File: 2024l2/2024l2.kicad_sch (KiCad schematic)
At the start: 124 parts, among them IC1 LM2587S-ADJ, J10 Conn_01x03, J11 Conn_01x04, J2 Conn_01x02, J4 Conn_01x02, J5 Conn_01x02, J7 Conn_01x03, J8 Conn_01x06, SW1 SW_SPST, U1 DRV8873SPWPRQ1, U3 TPS5430DDA, U4 TPS5430DDA, U7 Teensy 4.0

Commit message: LCSC Updates
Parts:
- C17, C3, C4: LCSC C577419 -> C3011705
- C29, C31: LCSC C5128349 -> C3011705
- D1, D2: LCSC C6807781 -> C85099
- R19: LCSC C22909 -> C137748
- R2: LCSC C25804 -> C21190
- R2: LCSC C25804 -> C23138
- R2: LCSC C25804 -> C21189
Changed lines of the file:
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@@
       (effects (font (size 1.27 1.27)) hide)
     )
-    (property "LCSC" "C25804" (at 281.94 49.53 0)
+    (property "LCSC" "C21190" (at 281.94 49.53 0)
       (effects (font (size 1.27 1.27)) hide)
     )
@@
       (effects (font (size 1.27 1.27)) hide)
     )
-    (property "LCSC" "C25804" (at 147.32 109.22 0)
+    (property "LCSC" "C21190" (at 147.32 109.22 0)
       (effects (font (size 1.27 1.27)) hide)
     )
@@
       (effects (font (size 1.27 1.27)) hide)
     )
-    (property "LCSC" "C577419" (at 255.27 34.29 0)
+    (property "LCSC" "C3011705" (at 255.27 34.29 0)
       (effects (font (size 1.27 1.27)) hide)
     )
@@
       (effects (font (size 1.27 1.27)) hide)
     )
-    (property "LCSC" "C25804" (at 281.94 115.57 0)
+    (property "LCSC" "C21190" (at 281.94 115.57 0)
       (effects (font (size 1.27 1.27)) hide)
     )
@@
       (effects (font (size 1.27 1.27)) hide)
     )
-    (property "LCSC" "C25804" (at 16.51 238.76 0)
+    (property "LCSC" "C23138" (at 16.51 238.76 0)
       (effects (font (size 1.27 1.27)) hide)
     )
@@
       (effects (font (size 1.27 1.27)) hide)
     )
-    (property "LCSC" "C25804" (at 222.25 116.84 0)
+    (property "LCSC" "C21189" (at 222.25 116.84 0)
       (effects (font (size 1.27 1.27)) hide)
     )
@@
       (effects (font (size 1.27 1.27)) hide)
     )
-    (property "LCSC" "C5128349" (at 331.47 191.77 0)
+    (property "LCSC" "C3011705" (at 331.47 191.77 0)
       (effects (font (size 1.27 1.27)) hide)
     )
@@
       (effects (font (size 1.27 1.27)) hide)
     )
-    (property "LCSC" "C25804" (at 356.87 123.19 0)
+    (property "LCSC" "C21189" (at 356.87 123.19 0)
       (effects (font (size 1.27 1.27)) hide)
     )
@@
       (effects (font (size 1.27 1.27)) hide)
     )
-    (property "LCSC" "C25804" (at 147.32 43.18 0)
+    (property "LCSC" "C21190" (at 147.32 43.18 0)
       (effects (font (size 1.27 1.27)) hide)
     )
@@
       (effects (font (size 1.27 1.27)) hide)
     )
-    (property "LCSC" "C6807781" (at 77.47 26.67 90)
+    (property "LCSC" "C85099" (at 77.47 26.67 90)
       (effects (font (size 1.27 1.27)) hide)
     )
@@
       (effects (font (size 1.27 1.27)) hide)
     )
-    (property "LCSC" "C577419" (at 106.68 72.39 0)
+    (property "LCSC" "C3011705" (at 106.68 72.39 0)
       (effects (font (size 1.27 1.27)) hide)
     )
@@
       (effects (font (size 1.27 1.27)) hide)
     )
-    (property "LCSC" "C25804" (at 222.25 50.8 0)
+    (property "LCSC" "C21189" (at 222.25 50.8 0)
       (effects (font (size 1.27 1.27)) hide)
     )
@@
       (effects (font (size 1.27 1.27)) hide)
     )
-    (property "LCSC" "C6807781" (at 77.47 72.39 90)
+    (property "LCSC" "C85099" (at 77.47 72.39 90)
       (effects (font (size 1.27 1.27)) hide)
     )
@@
       (effects (font (size 1.27 1.27)) hide)
     )
-    (property "LCSC" "C577419" (at 394.97 105.41 0)
+    (property "LCSC" "C3011705" (at 394.97 105.41 0)
       (effects (font (size 1.27 1.27)) hide)
     )
@@
       (effects (font (size 1.27 1.27)) hide)
     )
-    (property "LCSC" "C577419" (at 106.68 26.67 0)
+    (property "LCSC" "C3011705" (at 106.68 26.67 0)
       (effects (font (size 1.27 1.27)) hide)
     )
@@
       (effects (font (size 1.27 1.27)) hide)
     )
-    (property "LCSC" "C25804" (at 16.51 267.97 0)
+    (property "LCSC" "C23138" (at 16.51 267.97 0)
       (effects (font (size 1.27 1.27)) hide)
     )
@@
       (effects (font (size 1.27 1.27)) hide)
     )
-    (property "LCSC" "C5128349" (at 232.41 191.77 0)
+    (property "LCSC" "C3011705" (at 232.41 191.77 0)
       (effects (font (size 1.27 1.27)) hide)
     )
@@
       (effects (font (size 1.27 1.27)) hide)
     )
-    (property "LCSC" "C25804" (at 31.75 269.24 0)
+    (property "LCSC" "C23138" (at 31.75 269.24 0)
       (effects (font (size 1.27 1.27)) hide)
     )
@@
       (effects (font (size 1.27 1.27)) hide)
     )
-    (property "LCSC" "C25804" (at 31.75 238.76 0)
+    (property "LCSC" "C23138" (at 31.75 238.76 0)
       (effects (font (size 1.27 1.27)) hide)
     )
@@
       (effects (font (size 1.27 1.27)) hide)
     )
-    (property "LCSC" "C577419" (at 256.54 100.33 0)
+    (property "LCSC" "C3011705" (at 256.54 100.33 0)
       (effects (font (size 1.27 1.27)) hide)
     )
@@
       (effects (font (size 1.27 1.27)) hide)
     )
-    (property "LCSC" "C25804" (at 356.87 57.15 0)
+    (property "LCSC" "C21189" (at 356.87 57.15 0)
       (effects (font (size 1.27 1.27)) hide)
     )
@@
       (effects (font (size 1.27 1.27)) hide)
     )
-    (property "LCSC" "C22909" (at 256.54 196.85 0)
+    (property "LCSC" "C137748" (at 256.54 196.85 0)
       (effects (font (size 1.27 1.27)) hide)
     )
@@
       (effects (font (size 1.27 1.27)) hide)
     )
-    (property "LCSC" "C577419" (at 394.97 39.37 0)
+    (property "LCSC" "C3011705" (at 394.97 39.37 0)
       (effects (font (size 1.27 1.27)) hide)
     )

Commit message: LCSC
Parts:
- L3: LCSC C7461383 -> C2875750
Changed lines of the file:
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@@
       (effects (font (size 1.27 1.27)) hide)
     )
-    (property "LCSC" "C7461383" (at 279.4 175.26 90)
+    (property "LCSC" "C2875750" (at 279.4 175.26 90)
       (effects (font (size 1.27 1.27)) hide)
     )

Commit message: Move motor switch
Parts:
- RV1: LCSC C124590 -> C3151613
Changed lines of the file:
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@@
       (effects (font (size 1.27 1.27)) hide)
     )
-    (property "LCSC" "C124590" (at 304.8 193.04 90)
+    (property "LCSC" "C3151613" (at 304.8 193.04 90)
       (effects (font (size 1.27 1.27)) hide)
     )

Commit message: Changed Cap LCSC
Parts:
- C3: LCSC C259982 -> C5162352
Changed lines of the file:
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@@
       (effects (font (size 1.27 1.27)) hide)
     )
-    (property "LCSC" "C259982" (at 382.27 39.37 0)
+    (property "LCSC" "C5162352" (at 382.27 39.37 0)
       (effects (font (size 1.27 1.27)) hide)
     )
@@
       (effects (font (size 1.27 1.27)) hide)
     )
-    (property "LCSC" "C259982" (at 243.84 100.33 0)
+    (property "LCSC" "C5162352" (at 243.84 100.33 0)
       (effects (font (size 1.27 1.27)) hide)
     )
@@
       (effects (font (size 1.27 1.27)) hide)
     )
-    (property "LCSC" "C259982" (at 242.57 34.29 0)
+    (property "LCSC" "C5162352" (at 242.57 34.29 0)
       (effects (font (size 1.27 1.27)) hide)
     )
@@
       (effects (font (size 1.27 1.27)) hide)
     )
-    (property "LCSC" "C259982" (at 382.27 105.41 0)
+    (property "LCSC" "C5162352" (at 382.27 105.41 0)
       (effects (font (size 1.27 1.27)) hide)
     )

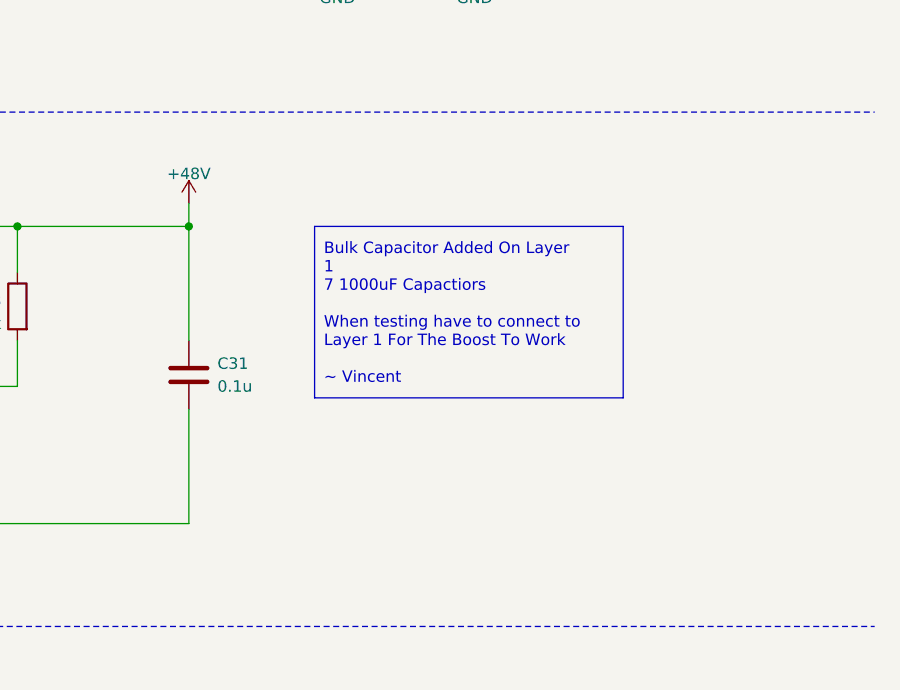
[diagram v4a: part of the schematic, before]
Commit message: Boost Caps
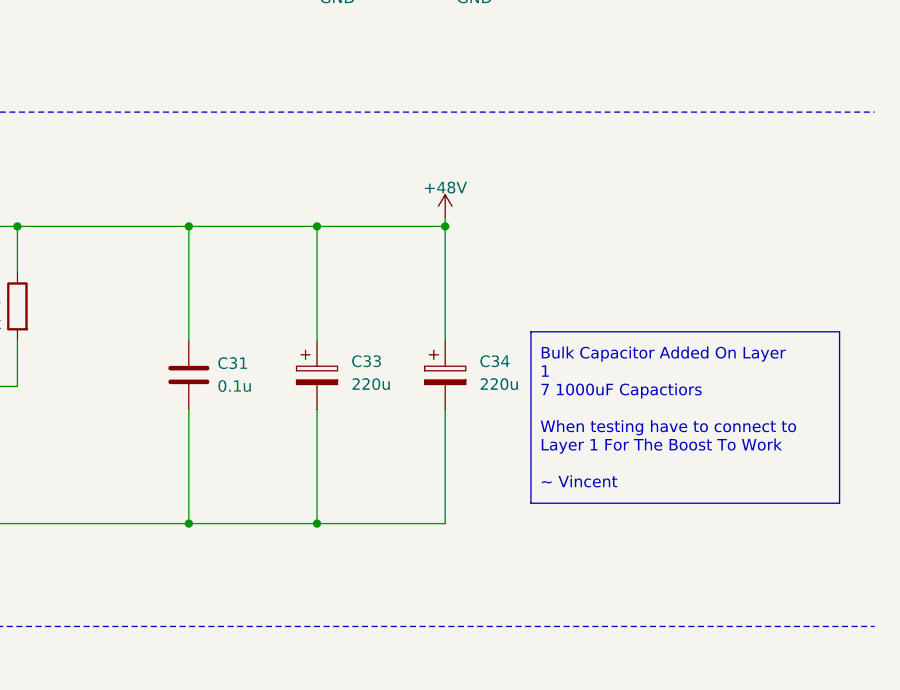
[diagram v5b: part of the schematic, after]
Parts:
- added C33, C34: 220u, Capacitor_SMD:CP_Elec_10x10.5, symbol Device:C_Polarized
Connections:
- net +48V: now also C33.1, C34.1
- net GND: now also C33.2, C34.2
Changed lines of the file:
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@@
   (junction (at 278.13 208.28) (diameter 0) (color 0 0 0 0)
   )
+  (junction (at 345.7119 175.26) (diameter 0) (color 0 0 0 0)
+  )
   (junction (at 347.98 105.41) (diameter 0) (color 0 0 0 0)
   )
@@
   (junction (at 228.6 138.43) (diameter 0) (color 0 0 0 0)
   )
+  (junction (at 359.9536 175.26) (diameter 0) (color 0 0 0 0)
+  )
   (junction (at 243.84 144.78) (diameter 0) (color 0 0 0 0)
   )
@@
   (junction (at 106.68 21.59) (diameter 0) (color 0 0 0 0)
   )
+  (junction (at 345.7119 208.28) (diameter 0) (color 0 0 0 0)
+  )
   (junction (at 92.71 67.31) (diameter 0) (color 0 0 0 0)
   )
@@
   (junction (at 299.72 193.04) (diameter 0) (color 0 0 0 0)
   )
+  (junction (at 331.47 208.28) (diameter 0) (color 0 0 0 0)
+  )
   (junction (at 331.47 175.26) (diameter 0) (color 0 0 0 0)
   )
@@
     (stroke (width 0) (type default))
   )
+  (wire (pts (xy 359.9536 175.26) (xy 359.9538 175.26))
+    (stroke (width 0) (type default))
+  )
   (polyline (pts (xy 12.7 102.87) (xy 127 102.87))
     (stroke (width 0) (type dash))
@@
     (stroke (width 0) (type default))
   )
+  (wire (pts (xy 331.47 208.28) (xy 345.7119 208.28))
+    (stroke (width 0) (type default))
+  )
   (wire (pts (xy 157.48 96.52) (xy 153.67 96.52))
     (stroke (width 0) (type default))
@@
     (stroke (width 0) (type default))
   )
-  (wire (pts (xy 331.47 175.26) (xy 331.47 172.72))
+  (wire (pts (xy 359.9536 175.26) (xy 359.9536 174.2915))
     (stroke (width 0) (type default))
   )
@@
     (stroke (width 0) (type default))
   )
+  (wire (pts (xy 345.7119 175.26) (xy 331.47 175.26))
+    (stroke (width 0) (type default))
+  )
+  (wire (pts (xy 345.7119 175.26) (xy 345.7119 188.0025))
+    (stroke (width 0) (type default))
+  )
   (wire (pts (xy 278.13 208.28) (xy 276.86 208.28))
     (stroke (width 0) (type default))
@@
     (stroke (width 0) (type default))
   )
+  (wire (pts (xy 359.9538 175.26) (xy 359.9538 188.0025))
+    (stroke (width 0) (type default))
+  )
   (wire (pts (xy 255.27 27.94) (xy 255.27 30.48))
     (stroke (width 0) (type default))
@@
     (stroke (width 0) (type default))
   )
+  (wire (pts (xy 345.7119 175.26) (xy 359.9536 175.26))
+    (stroke (width 0) (type default))
+  )
   (wire (pts (xy 299.72 71.12) (xy 309.88 71.12))
     (stroke (width 0) (type default))
@@
     (stroke (width 0) (type default))
   )
+  (wire (pts (xy 345.7119 208.28) (xy 359.9538 208.28))
+    (stroke (width 0) (type default))
+  )
   (wire (pts (xy 77.47 76.2) (xy 77.47 77.47))
     (stroke (width 0) (type default))
@@
     (stroke (width 0) (type default))
   )
+  (wire (pts (xy 359.9538 208.28) (xy 359.9538 195.6225))
+    (stroke (width 0) (type default))
+  )
   (wire (pts (xy 299.72 55.88) (xy 309.88 55.88))
     (stroke (width 0) (type default))
@@
     (stroke (width 0) (type default))
   )
+  (wire (pts (xy 345.7119 208.28) (xy 345.7119 195.6225))
+    (stroke (width 0) (type default))
+  )
   (wire (pts (xy 213.36 87.63) (xy 213.36 90.17))
     (stroke (width 0) (type default))
@@
   )
   (text_box "Bulk Capacitor Added On Layer 1\n7 1000uF Capactiors\n\nWhen testing have to connect to Layer 1 For The Boost To Work\n\n~ Vincent"
-    (at 345.44 175.26 0) (size 34.29 19.05)
+    (at 369.4814 186.9696 0) (size 34.29 19.05)
     (stroke (width 0) (type default))
     (fill (type none))
@@
     )
   )
+  (symbol (lib_id "Device:C_Polarized") (at 345.7119 191.8125 0) (unit 1)
+    (in_bom yes) (on_board yes) (dnp no) (fields_autoplaced)
+    (property "Reference" "C33" (at 349.5219 190.2885 0)
+      (effects (font (size 1.27 1.27)) (justify left))
+    )
+    (property "Value" "220u" (at 349.5219 192.8285 0)
+      (effects (font (size 1.27 1.27)) (justify left))
+    )
+    (property "Footprint" "Capacitor_SMD:CP_Elec_10x10.5" (at 346.6771 195.6225 0)
+      (effects (font (size 1.27 1.27)) hide)
+    )
+    (property "Datasheet" "~" (at 345.7119 191.8125 0)
+      (effects (font (size 1.27 1.27)) hide)
+    )
+    (property "LCSC" "C7471900" (at 345.7119 191.8125 0)
+      (effects (font (size 1.27 1.27)) hide)
+    )
+    (pin "1")
+    (pin "2")
+    (instances
+      (project "2024l2"
+        (path "/36f2ccec-186b-4304-87fe-6495d5655b87"
+          (reference "C33") (unit 1)
+        )
+      )
+      (project "2024l1"
+        (path "/5be543b5-1bdc-438f-a916-f916127c0a2b"
+          (reference "C?") (unit 1)
+        )
+      )
+      (project "2023l1-int"
+        (path "/dd82140d-c14c-4d8d-8674-edeceaca486e"
+          (reference "C?") (unit 1)
+        )
+      )
+      (project "buck"
+        (path "/df3073b9-8d60-44a4-89ea-71f9aa763c80"
+          (reference "C?") (unit 1)
+        )
+      )
+    )
+  )
   (symbol (lib_id "Connector_Generic:Conn_01x03") (at 49.53 133.35 180) (unit 1)
     (in_bom yes) (on_board yes) (dnp no)
@@
     )
   )
+  (symbol (lib_id "Device:C_Polarized") (at 359.9538 191.8125 0) (unit 1)
+    (in_bom yes) (on_board yes) (dnp no) (fields_autoplaced)
+    (property "Reference" "C34" (at 363.7638 190.2885 0)
+      (effects (font (size 1.27 1.27)) (justify left))
+    )
+    (property "Value" "220u" (at 363.7638 192.8285 0)
+      (effects (font (size 1.27 1.27)) (justify left))
+    )
+    (property "Footprint" "Capacitor_SMD:CP_Elec_10x10.5" (at 360.919 195.6225 0)
+      (effects (font (size 1.27 1.27)) hide)
+    )
+    (property "Datasheet" "~" (at 359.9538 191.8125 0)
+      (effects (font (size 1.27 1.27)) hide)
+    )
+    (property "LCSC" "C7471900" (at 359.9538 191.8125 0)
+      (effects (font (size 1.27 1.27)) hide)
+    )
+    (pin "1")
+    (pin "2")
+    (instances
+      (project "2024l2"
+        (path "/36f2ccec-186b-4304-87fe-6495d5655b87"
+          (reference "C34") (unit 1)
+        )
+      )
+      (project "2024l1"
+        (path "/5be543b5-1bdc-438f-a916-f916127c0a2b"
+          (reference "C?") (unit 1)
+        )
+      )
+      (project "2023l1-int"
+        (path "/dd82140d-c14c-4d8d-8674-edeceaca486e"
+          (reference "C?") (unit 1)
+        )
+      )
+      (project "buck"
+        (path "/df3073b9-8d60-44a4-89ea-71f9aa763c80"
+          (reference "C?") (unit 1)
+        )
+      )
+    )
+  )
   (symbol (lib_id "Device:D_Schottky") (at 303.53 175.26 180) (unit 1)
     (in_bom yes) (on_board yes) (dnp no) (fields_autoplaced)
@@
     )
   )
-  (symbol (lib_id "power:+48V") (at 331.47 172.72 0) (unit 1)
+  (symbol (lib_id "power:+48V") (at 359.9536 174.2915 0) (unit 1)
     (in_bom yes) (on_board yes) (dnp no)
-    (property "Reference" "#PWR078" (at 331.47 176.53 0)
+    (property "Reference" "#PWR078" (at 359.9536 178.1015 0)
       (effects (font (size 1.27 1.27)) hide)
     )
-    (property "Value" "+48V" (at 331.47 169.418 0)
+    (property "Value" "+48V" (at 359.9536 170.9895 0)
       (effects (font (size 1.27 1.27)))
     )
-    (property "Footprint" "" (at 331.47 172.72 0)
+    (property "Footprint" "" (at 359.9536 174.2915 0)
       (effects (font (size 1.27 1.27)) hide)
     )
-    (property "Datasheet" "" (at 331.47 172.72 0)
+    (property "Datasheet" "" (at 359.9536 174.2915 0)
       (effects (font (size 1.27 1.27)) hide)
     )

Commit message: L2
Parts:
- C30: footprint Capacitor_SMD:CP_Elec_8x10.5 -> Capacitor_SMD:CP_Elec_8x6.5; LCSC C5355007 -> C249586
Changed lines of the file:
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@@
       (effects (font (size 1.27 1.27)) (justify left))
     )
-    (property "Footprint" "Capacitor_SMD:CP_Elec_8x10.5" (at 246.0752 195.58 0)
+    (property "Footprint" "Capacitor_SMD:CP_Elec_8x6.5" (at 246.0752 195.58 0)
       (effects (font (size 1.27 1.27)) hide)
     )
@@
       (effects (font (size 1.27 1.27)) hide)
     )
-    (property "LCSC" "C5355007" (at 245.11 191.77 0)
+    (property "LCSC" "C249586" (at 245.11 191.77 0)
       (effects (font (size 1.27 1.27)) hide)
     )
